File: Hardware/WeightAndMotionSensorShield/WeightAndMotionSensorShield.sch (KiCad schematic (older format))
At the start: 19 parts, among them J1 PIR, J2 CELLS, J3 UL, J4 LL, J5 CELLS, J6 UR, J7 LR, P1 Power, P2 Analog, P3 Digital, P4 Digital, P5 CONN_01X01, P6 CONN_01X01, P7 CONN_01X01, P8 CONN_01X01, SW1 RESET, U1 HX711_PCB

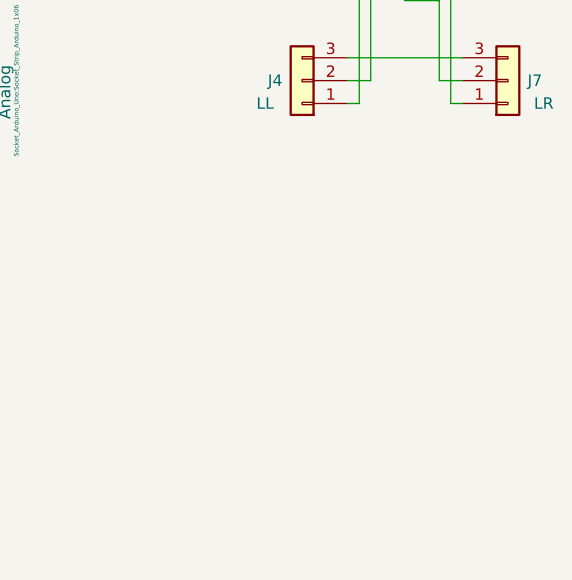
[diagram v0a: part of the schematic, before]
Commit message: PCB v1.1 and 2 changes
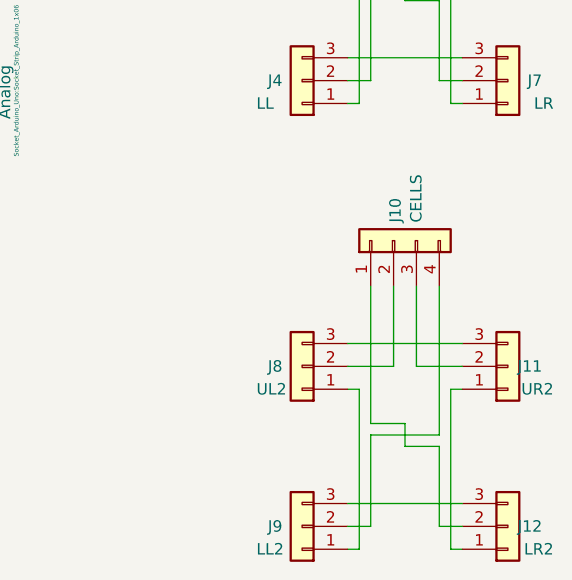
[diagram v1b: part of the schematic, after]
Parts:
- added J10: CELLS, Connector_PinHeader_2.54mm:PinHeader_1x04_P2.54mm_Vertical, symbol Connector_Generic:Conn_01x04
- added J11: UR2, Connector_PinHeader_2.54mm:PinHeader_1x03_P2.54mm_Vertical, symbol Connector_Generic:Conn_01x03
- added J12: LR2, Connector_PinHeader_2.54mm:PinHeader_1x03_P2.54mm_Vertical, symbol Connector_Generic:Conn_01x03
- added J8: UL2, Connector_PinSocket_2.54mm:PinSocket_1x03_P2.54mm_Vertical, symbol Connector_Generic:Conn_01x03
- added J9: LL2, Connector_PinHeader_2.54mm:PinHeader_1x03_P2.54mm_Vertical, symbol Connector_Generic:Conn_01x03
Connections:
- new net: J11.1 (Pin_1), J12.1 (Pin_1)
- new net: J10.1 (Pin_1), J12.2 (Pin_2)
- new net: J12.3 (Pin_3), J9.3 (Pin_3)
- new net: J8.1 (Pin_1), J9.1 (Pin_1)
- new net: J10.4 (Pin_4), J9.2 (Pin_2)
- new net: J10.3 (Pin_3), J11.2 (Pin_2)
- new net: J11.3 (Pin_3), J8.3 (Pin_3)
- new net: J10.2 (Pin_2), J8.2 (Pin_2)
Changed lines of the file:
@@
 Wire Wire Line
 	4300 3800 5100 3800
+$Comp
+L Connector_Generic:Conn_01x03 J12
+U 1 1 5D3800F0
+P 10250 6100
+F 0 "J12" H 10400 6100 50  0000 R CNN
+F 1 "LR2" H 10450 6200 50  0000 R CNN
+F 2 "Connector_PinHeader_2.54mm:PinHeader_1x03_P2.54mm_Vertical" H 10250 6100 50  0001 C CNN
+F 3 "~" H 10250 6100 50  0001 C CNN
+	1    10250 6100
+	1    0    0    1
+$EndComp
+$Comp
+L Connector_Generic:Conn_01x03 J9
+U 1 1 5D3800F7
+P 9350 6100
+F 0 "J9" H 9500 6100 50  0000 R CNN
+F 1 "LL2" H 9550 6200 50  0000 R CNN
+F 2 "Connector_PinHeader_2.54mm:PinHeader_1x03_P2.54mm_Vertical" H 9350 6100 50  0001 C CNN
+F 3 "~" H 9350 6100 50  0001 C CNN
+	1    9350 6100
+	-1   0    0    1
+$EndComp
+$Comp
+L Connector_Generic:Conn_01x03 J11
+U 1 1 5D3800FE
+P 10250 5400
+F 0 "J11" H 10400 5400 50  0000 R CNN
+F 1 "UR2" H 10450 5500 50  0000 R CNN
+F 2 "Connector_PinHeader_2.54mm:PinHeader_1x03_P2.54mm_Vertical" H 10250 5400 50  0001 C CNN
+F 3 "~" H 10250 5400 50  0001 C CNN
+	1    10250 5400
+	1    0    0    1
+$EndComp
+$Comp
+L Connector_Generic:Conn_01x03 J8
+U 1 1 5D380105
+P 9350 5400
+F 0 "J8" H 9500 5400 50  0000 R CNN
+F 1 "UL2" H 9550 5500 50  0000 R CNN
+F 2 "Connector_PinSocket_2.54mm:PinSocket_1x03_P2.54mm_Vertical" H 9350 5400 50  0001 C CNN
+F 3 "~" H 9350 5400 50  0001 C CNN
+	1    9350 5400
+	-1   0    0    1
+$EndComp
+$Comp
+L Connector_Generic:Conn_01x04 J10
+U 1 1 5D38010C
+P 9750 4850
+F 0 "J10" H 9829 4842 50  0000 L CNN
+F 1 "CELLS" H 9829 4751 50  0000 L CNN
+F 2 "Connector_PinHeader_2.54mm:PinHeader_1x04_P2.54mm_Vertical" H 9750 4850 50  0001 C CNN
+F 3 "~" H 9750 4850 50  0001 C CNN
+	1    9750 4850
+	0    -1   -1   0
+$EndComp
+Wire Wire Line
+	9750 5400 9750 5050
+Wire Wire Line
+	9850 5400 9850 5050
+Wire Wire Line
+	9550 5400 9750 5400
+Wire Wire Line
+	9850 5400 10050 5400
+Wire Wire Line
+	9950 5700 9950 5050
+Wire Wire Line
+	9800 5650 9650 5650
+Wire Wire Line
+	9650 5650 9650 5050
+Wire Wire Line
+	9550 6100 9650 6100
+Wire Wire Line
+	9650 5700 9650 6100
+Wire Wire Line
+	9650 5700 9950 5700
+Wire Wire Line
+	9950 6100 10050 6100
+Wire Wire Line
+	9800 5650 9800 5750
+Wire Wire Line
+	9800 5750 9950 5750
+Wire Wire Line
+	9950 5750 9950 6100
+Wire Wire Line
+	9550 5300 10050 5300
+Wire Wire Line
+	9550 5500 9600 5500
+Wire Wire Line
+	9600 5500 9600 6200
+Wire Wire Line
+	9600 6200 9550 6200
+Wire Wire Line
+	10050 6200 10000 6200
+Wire Wire Line
+	10000 6200 10000 5500
+Wire Wire Line
+	10000 5500 10050 5500
+Wire Wire Line
+	9550 6000 10050 6000
 $EndSCHEMATC
